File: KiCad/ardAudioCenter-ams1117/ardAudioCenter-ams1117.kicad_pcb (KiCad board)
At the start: 2 copper layers, 99.7 x 66 mm, 24 parts, among them J1 2-pin_power_input_header, J3 4-pin_I2C_LCD_header, U1 2-pole_power_in_screw_terminal, U10 CD4052B, U11 MCP41010, U13 4-pole_RL-input_screw_terminal, U15 TEA5767_FM_Radio_Module, U16 VolR, U2 KY-040_Rotary_Encoder, U3 AMS1117-5.0, U5 KY-040_Rotary_Encoder, U6 JDY-62_Bluetooth_Module, U7 4-pole_RL-output_screw_termin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, U8 MCP41010, U9 VolL

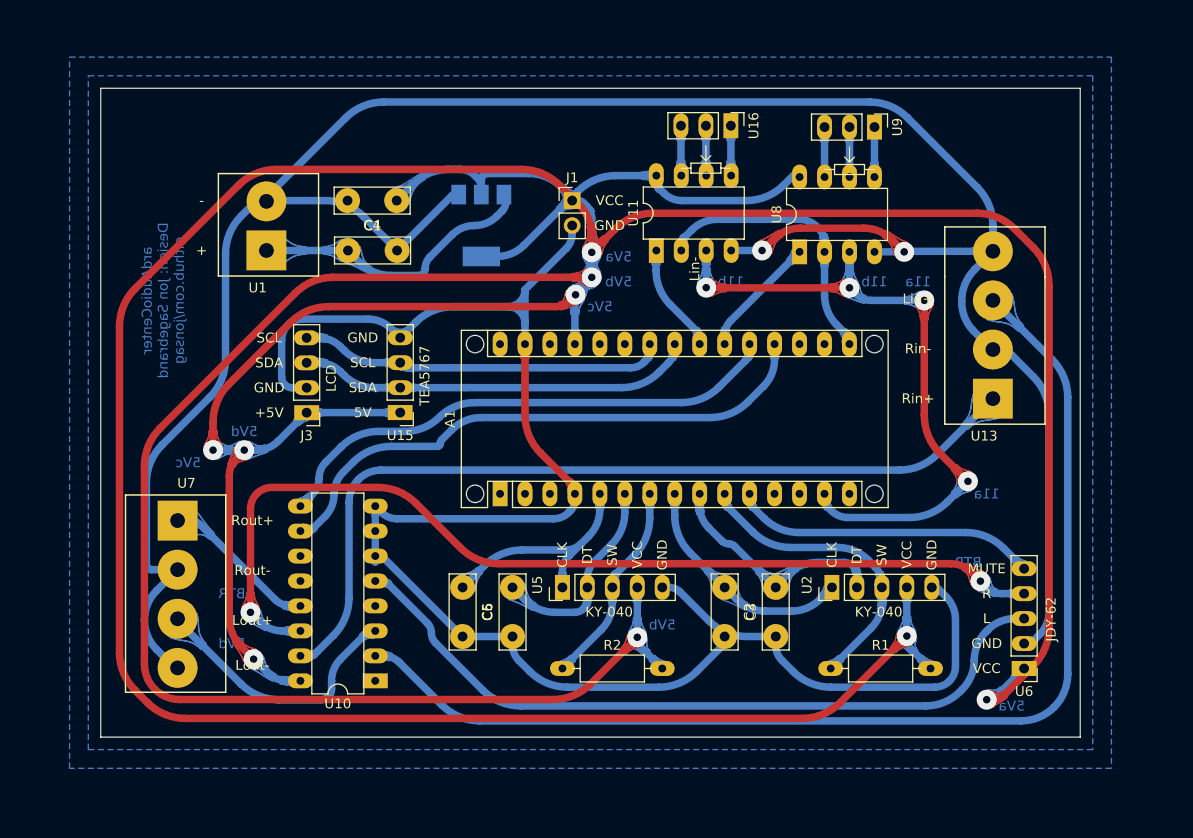
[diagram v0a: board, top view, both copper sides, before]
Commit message: 2-layer PCB
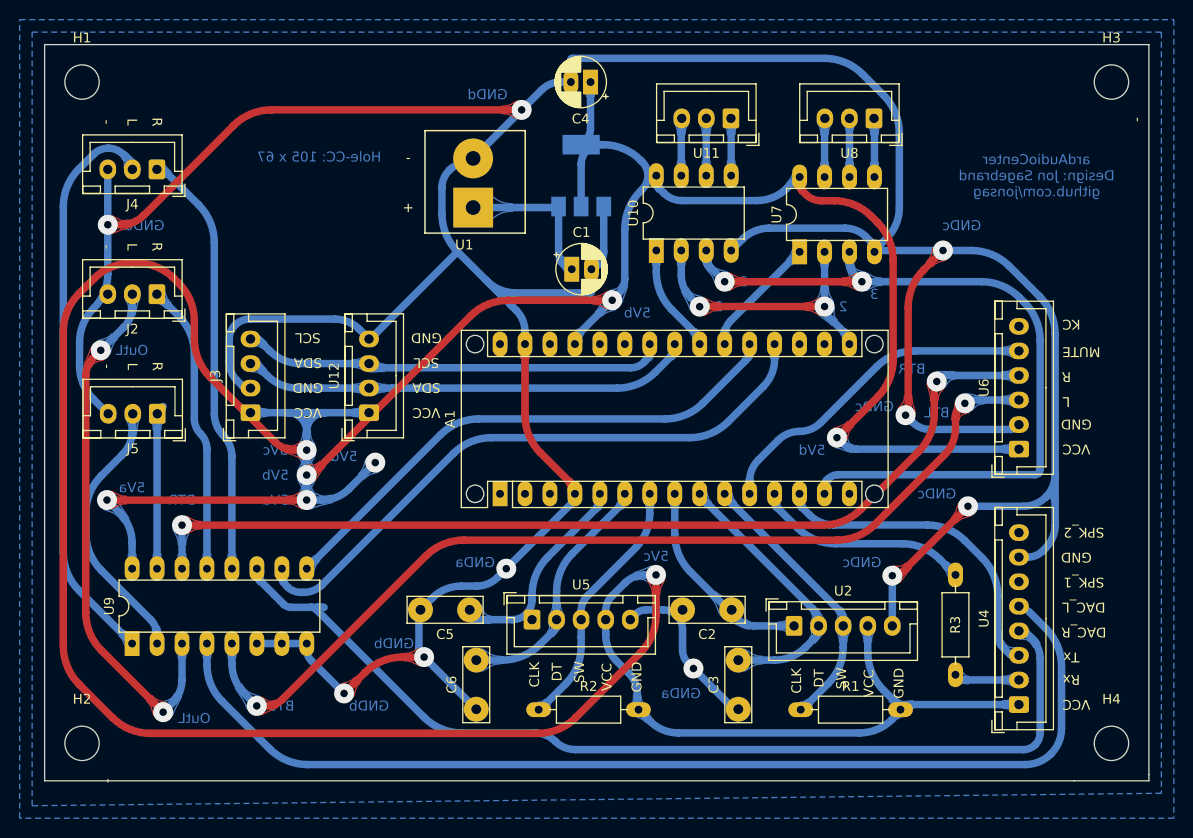
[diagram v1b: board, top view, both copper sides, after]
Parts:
- removed J1: 2-pin_power_input_header, My_Headers:2-pin_power_input_header
- removed U13: 4-pole_RL-input_screw_terminal, My_Parts:4-pole_screw_terminal_RL_input
- removed U15: TEA5767_FM_Radio_Module, My_Headers:4-pin_TEA5767_radio_module_header_large
- removed the U7 at (80.2, 80.8)
- added H1: MountingHole, MountingHole:MountingHole_3.5mm, F.Cu at (70.5, 36.2)
- added H2: MountingHole, MountingHole:MountingHole_3.5mm, F.Cu at (70.5, 103.5)
- added H3: MountingHole, MountingHole:MountingHole_3.5mm, F.Cu at (175.3, 36.2)
- added H4: MountingHole, MountingHole:MountingHole_3.5mm, F.Cu at (175.3, 103.5)
- added J2: Audio out, My_Headers:3-pin JST Audio, F.Cu at (78.1, 57.8)
- added J4: FM In, My_Headers:3-pin JST Audio, F.Cu at (78.1, 45.1)
- added J5: Line In, My_Headers:3-pin JST Audio, F.Cu at (78.1, 70.0)
- added R3: 330R, My_Misc:R_Axial_DIN0207_L6.3mm_D2.5mm_P10.16mm_Horizontal_larger_pads, F.Cu at (159.4, 96.5)
- added U12: FM Radio, My_Headers:4-pin JST TEA5767 FM Radio, F.Cu at (99.7, 69.8)
- added U4: DFPlayer_Mini, My_Headers:8-pin JST DFPlayer Mini, F.Cu at (165.8, 99.6)
- C1: value 0.33u -> 10u; footprint My_Misc:C_Disc_D7.5mm_W2.5mm_P5.00mm_larger -> My_Misc:CP_Radial_D5.0mm_P2.00mm_larger
- C4: value 0.1u -> 22u; footprint My_Misc:C_Disc_D7.5mm_W2.5mm_P5.00mm_larger -> My_Misc:CP_Radial_D5.0mm_P2.00mm_larger
- J3: value 4-pin_I2C_LCD_header -> LCD; footprint My_Headers:4-pin_I2C_LCD_header_larger -> My_Headers:4-pin JST LCD
- U11: renamed from U16; footprint My_Headers:3-pin_potentiometer_header_larger_pads -> My_Misc:JST_XH_B3B-XH-A_1x03_P2.50mm_Vertical large
- U2: value KY-040_Rotary_Encoder -> Rotary encoder 2; footprint My_Headers:5-pin_KY-040_rotary_encoder_header_larger -> My_Headers:5-pin JST Rotary Encoder
- U5: value KY-040_Rotary_Encoder -> Rotary encoder 1; footprint My_Headers:5-pin_KY-040_rotary_encoder_header_larger -> My_Headers:5-pin JST Rotary Encoder
- U6: footprint My_Headers:5-pin_JDY-62_bluetooth_module_header_large -> My_Headers:6-pin JST JDY-62 Bluetooth
- U8: renamed from U9; footprint My_Headers:3-pin_potentiometer_header_larger_pads -> My_Misc:JST_XH_B3B-XH-A_1x03_P2.50mm_Vertical large
- moved U9 25.0 mm to (75.6, 93.3), turned to 90 degrees
- moved C4 23.1 mm to (122.2, 36.2)
- moved C1 22.9 mm to (120.3, 55.2)
- moved U6 22.3 mm to (165.8, 73.6), turned to 90 degrees
- moved U1 21.5 mm to (110.3, 49.0)
- moved U3 11.4 mm to (121.3, 45.7), turned to 90 degrees
- moved C3 8.33 mm to (137.3, 100.0)
- moved C6 8.27 mm to (110.6, 100.0)
- moved J3 5.72 mm to (87.6, 69.8), turned to 90 degrees
- moved U2 5.50 mm to (143.0, 91.5), turned to 0 degrees
- moved R1 5.18 mm to (143.6, 100.1)
- moved R2 4.84 mm to (117.0, 100.1)
- moved U5 4.51 mm to (116.3, 90.9), turned to 0 degrees
- moved C2 2.39 mm to (136.6, 89.9), turned to 180 degrees
- moved C5 2.39 mm to (109.9, 89.9), turned to 180 degrees
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- renumbered U11 to U10, U8 to U7, U10 to U9
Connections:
- J3 pad 3: GND -> /SDA
- U9 pad 1: FML+ -> Net-(J4-Pad2)
- U9 pad 12: FMR+ -> Net-(J4-Pad1)
- U9 pad 15: LineR+ -> Net-(J5-Pad1)
- U9 pad 2: LineL+ -> Net-(J5-Pad2)
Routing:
- net +5V: track 602.7 -> 424.6 mm, vias 9 -> 8
- net LineL+: track 116.5 -> 0.00 mm
- net SDL+: track 0.00 -> 109.2 mm
- net SDR+: track 0.00 -> 100.7 mm
- net LineR+: track 88.2 -> 0.00 mm
- net Net-(J4-Pad2): track 0.00 -> 59.2 mm
- net Net-(J4-Pad1): track 0.00 -> 43.9 mm
- net /DFP-Tx: track 0.00 -> 32.9 mm
- net Net-(J5-Pad2): track 0.00 -> 27.6 mm
- net /Lout+: track 27.6 -> 54.9 mm, vias 0 -> 2
- net BTL+: track 77.1 -> 99.0 mm, vias 0 -> 2
- net Net-(A1-Pad12): track 0.00 -> 21.9 mm
- net Net-(J5-Pad1): track 0.00 -> 16.7 mm
- net +12V: track 29.4 -> 15.2 mm
- net /Rout+: track 16.2 -> 29.6 mm
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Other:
- board size 99.7 x 66 mm -> 112.4 x 74.9 mm
- board text added: "-"
- board text added: "2"
- board text added: "3"
- board text added: "BTL"
- board text added: "GNDa"
- board text added: "GNDb"
- board text added: "GNDc"
- board text added: "GNDd"
- board text added: "Hole-CC: 105 x 67"
- board text added: "OutL"
- board text removed: "11a"
- board text removed: "11b"
